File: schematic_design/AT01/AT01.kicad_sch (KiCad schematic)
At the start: 52 parts, among them J1 JST Connector, J2 Conn_01x08, J3 USB_C_Receptacle_USB2.0, J4 DC Pump Connector, J5 Solenoid Valve Connector, Q1 DMG2301L, Q2 2N7002, Q3 2N7002, SW1 SW_Push, SW2 SW_Push, SW3 SW_Push, U1 MPRLS0025PA00001A, U2 FT232RL, U3 DRV8833PW, U4 MCP73831-2-OT, U5 ESP32-WROOM-32, U6 LM1117MP-3.3

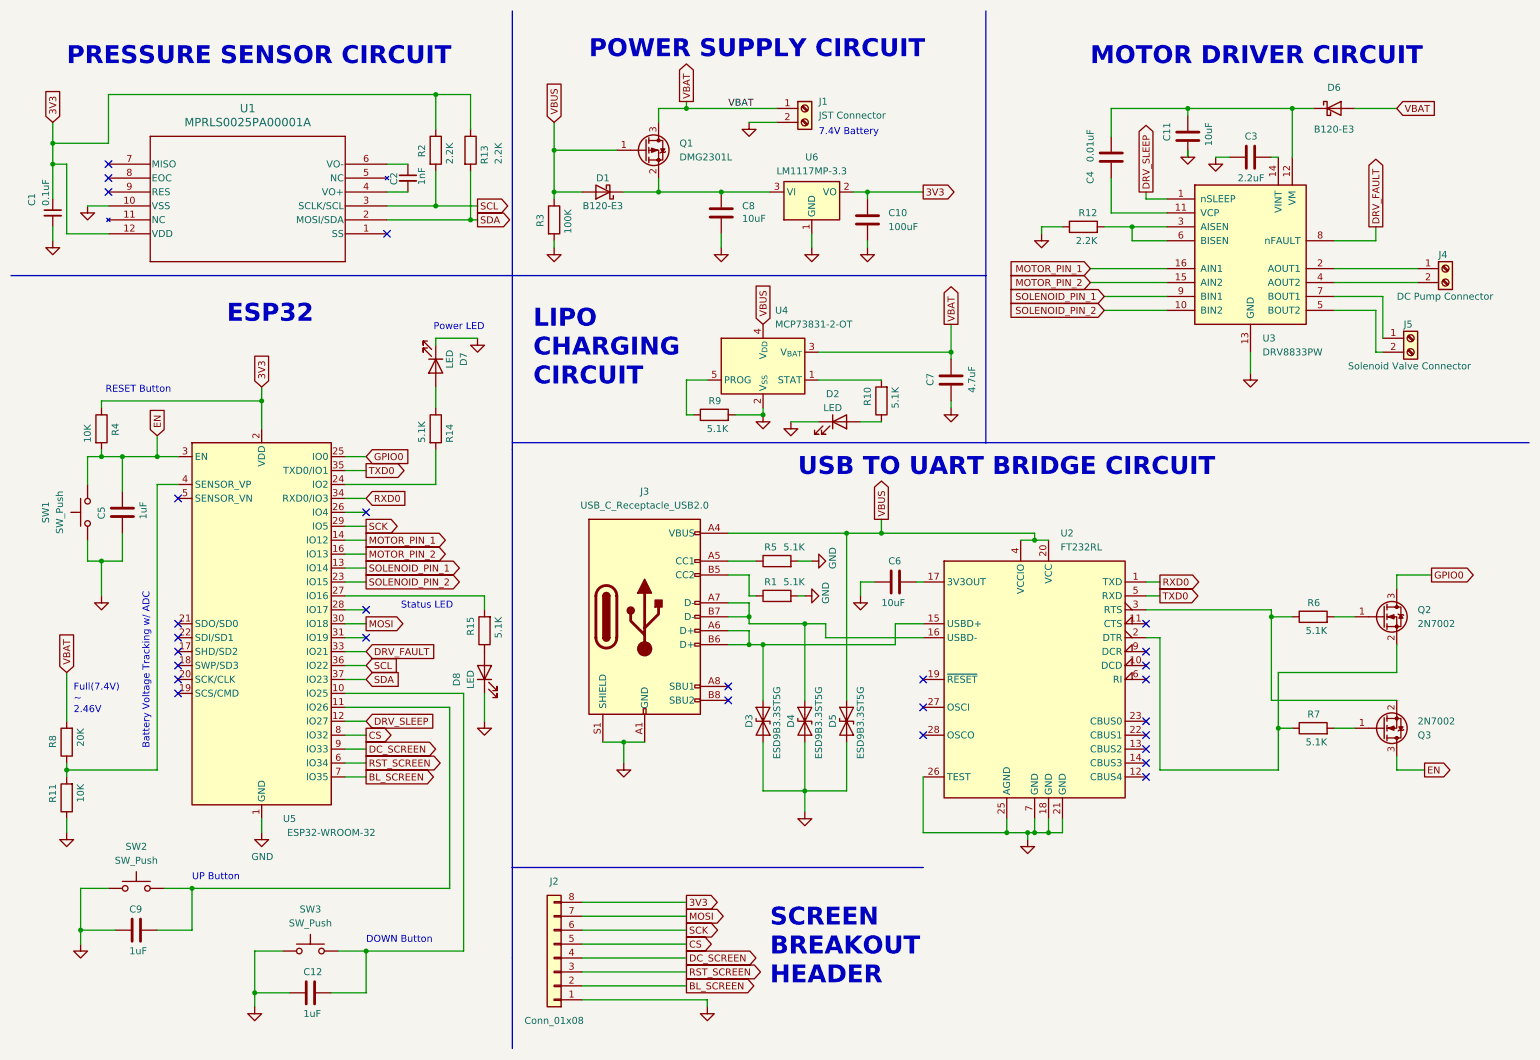
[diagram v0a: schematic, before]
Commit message: initial layout revision
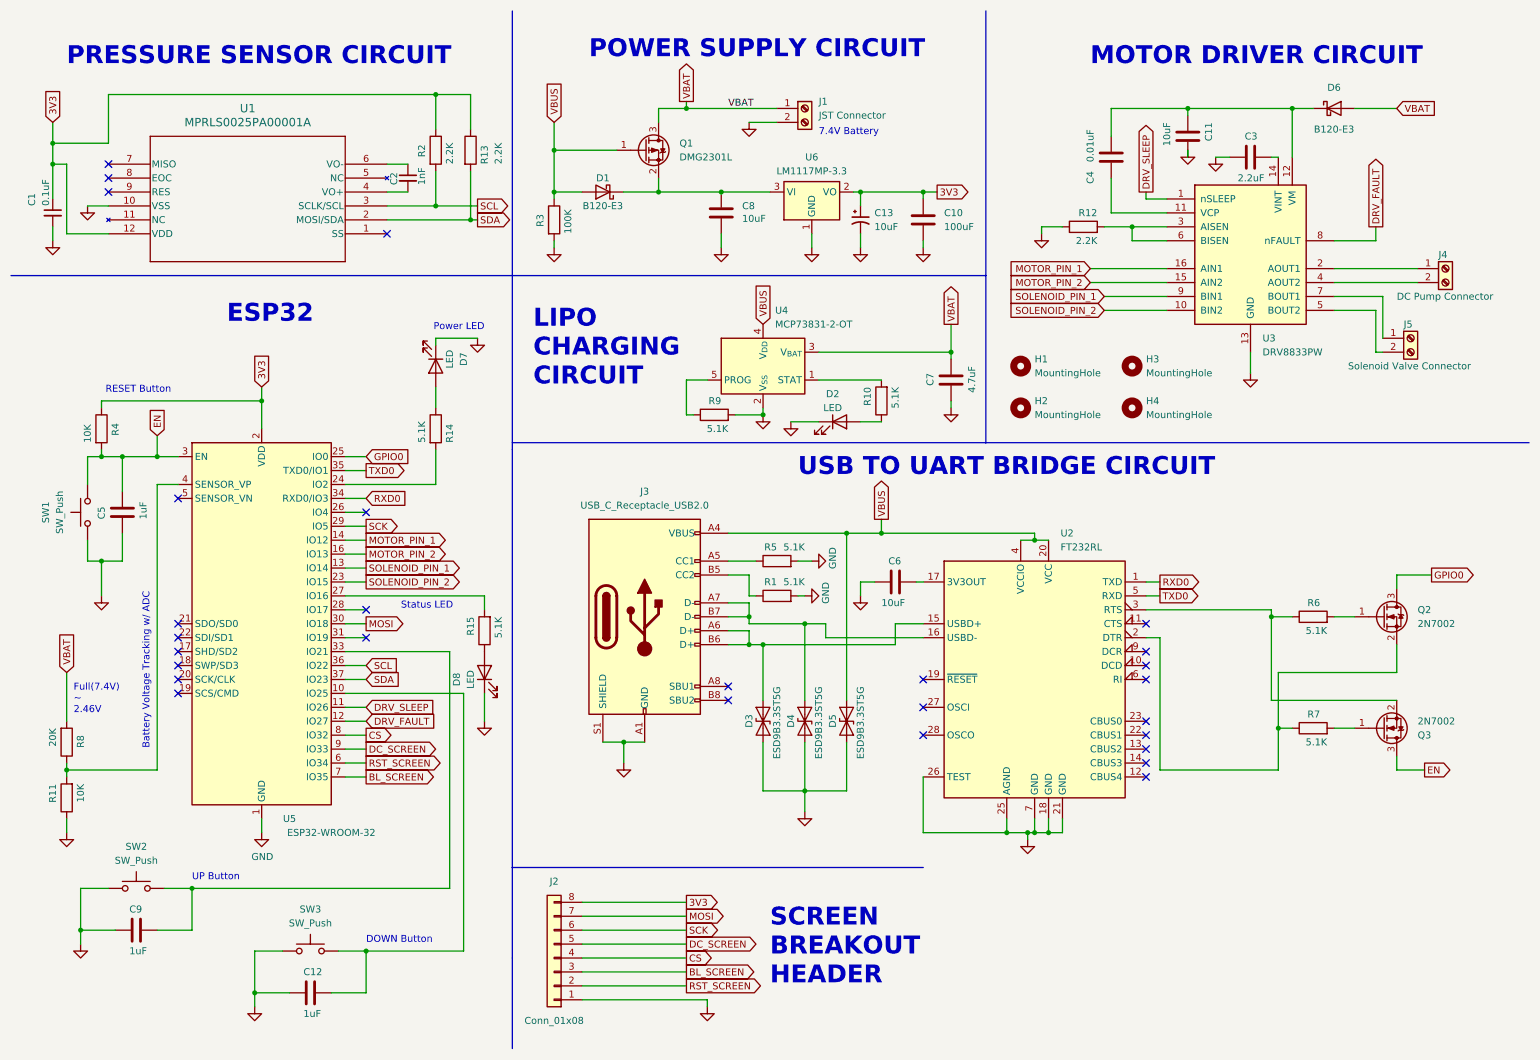
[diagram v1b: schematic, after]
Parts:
- added C13: 10uF, Capacitor_SMD:C_1206_3216Metric_Pad1.33x1.80mm_HandSolder, symbol Device:C_Polarized_Small_US
- added H1, H2, H3, H4: MountingHole, MountingHole:MountingHole_2.2mm_M2_ISO7380, symbol Mechanical:MountingHole
- C1, C10, C11, C12, C2, C3, C4, C5, C6, C7, C8, C9: footprint Capacitor_SMD:C_01005_0402Metric_Pad0.57x0.30mm_HandSolder -> Capacitor_SMD:C_0402_1005Metric_Pad0.74x0.62mm_HandSolder
- J3: footprint Connector_USB:USB_C_Receptacle_Molex_105450-0101 -> Connector_USB:USB_C_Receptacle_HRO_TYPE-C-31-M-12
- U5: footprint RF_Module:ESP32-WROOM-32D -> RF_Module:ESP32-WROOM-32U; symbol RF_Module:ESP32-WROOM-32D -> RF_Module:ESP32-WROOM-32U
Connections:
- net 3V3: now also C13.1
- net BL_SCREEN: now also J2.3 (Pin_3); no longer J2.2 (Pin_2)
- net CS: now also J2.4 (Pin_4); no longer J2.5 (Pin_5)
- net DC_SCREEN: now also J2.5 (Pin_5); no longer J2.4 (Pin_4)
- net DRV_FAULT: now also U5.12 (IO27); no longer U5.33 (IO21)
- net DRV_SLEEP: now also U5.11 (IO26); no longer U5.12 (IO27)
- net GND: now also C13.2
- net RST_SCREEN: now also J2.2 (Pin_2); no longer J2.3 (Pin_3)
- net at C9.1, SW2.1: now also U5.33 (IO21); no longer U5.11 (IO26)
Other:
- moved on the sheet: C10, C11, R8
